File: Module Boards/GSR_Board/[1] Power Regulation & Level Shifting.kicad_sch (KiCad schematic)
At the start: 25 parts, among them U5 TPS7A9401DSCR, U6 TXS0102DQER

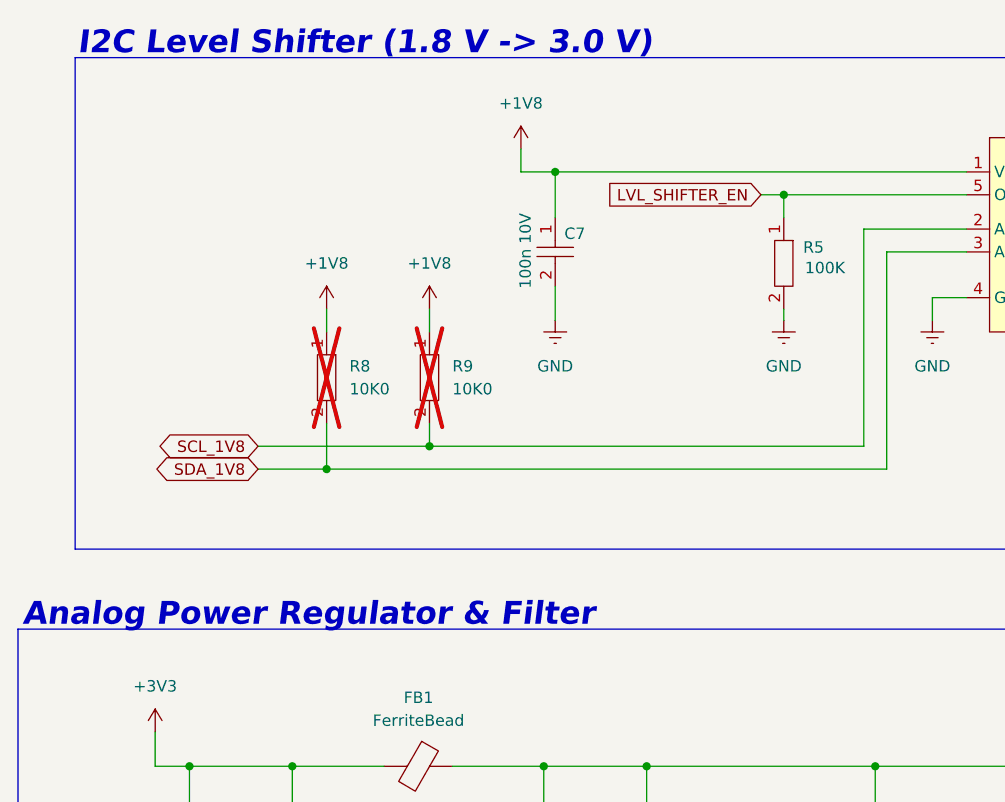
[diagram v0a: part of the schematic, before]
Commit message: Finished Routing of GSR Board
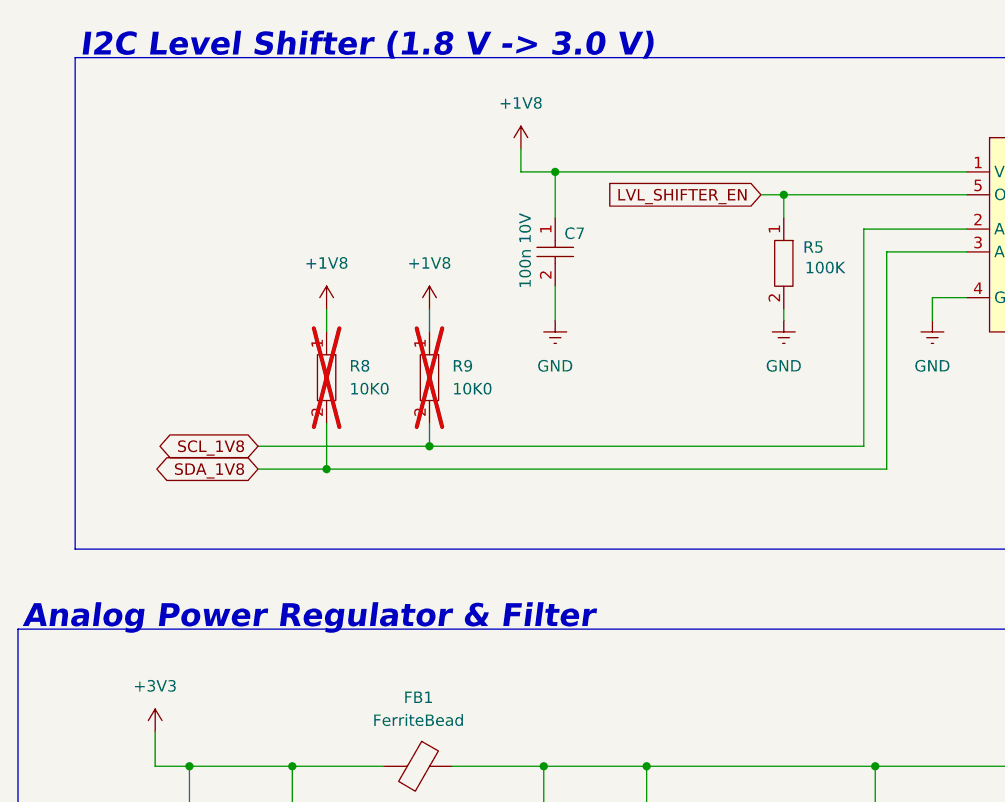
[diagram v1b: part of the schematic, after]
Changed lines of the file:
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@@
 	(text "I2C Level Shifter (1.8 V -> 3.0 V)"
 		(exclude_from_sim no)
-		(at 51.054 28.956 0)
+		(at 51.308 29.21 0)
 		(effects
 			(font
@@
 	(text "Analog Power Regulator & Filter"
 		(exclude_from_sim no)
-		(at 44.958 92.456 0)
+		(at 44.958 92.71 0)
 		(effects
 			(font
